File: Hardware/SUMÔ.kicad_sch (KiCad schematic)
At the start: 17 parts, among them M1 Motor_DC, M2 Motor_DC, SW1 SW_DPST_x2

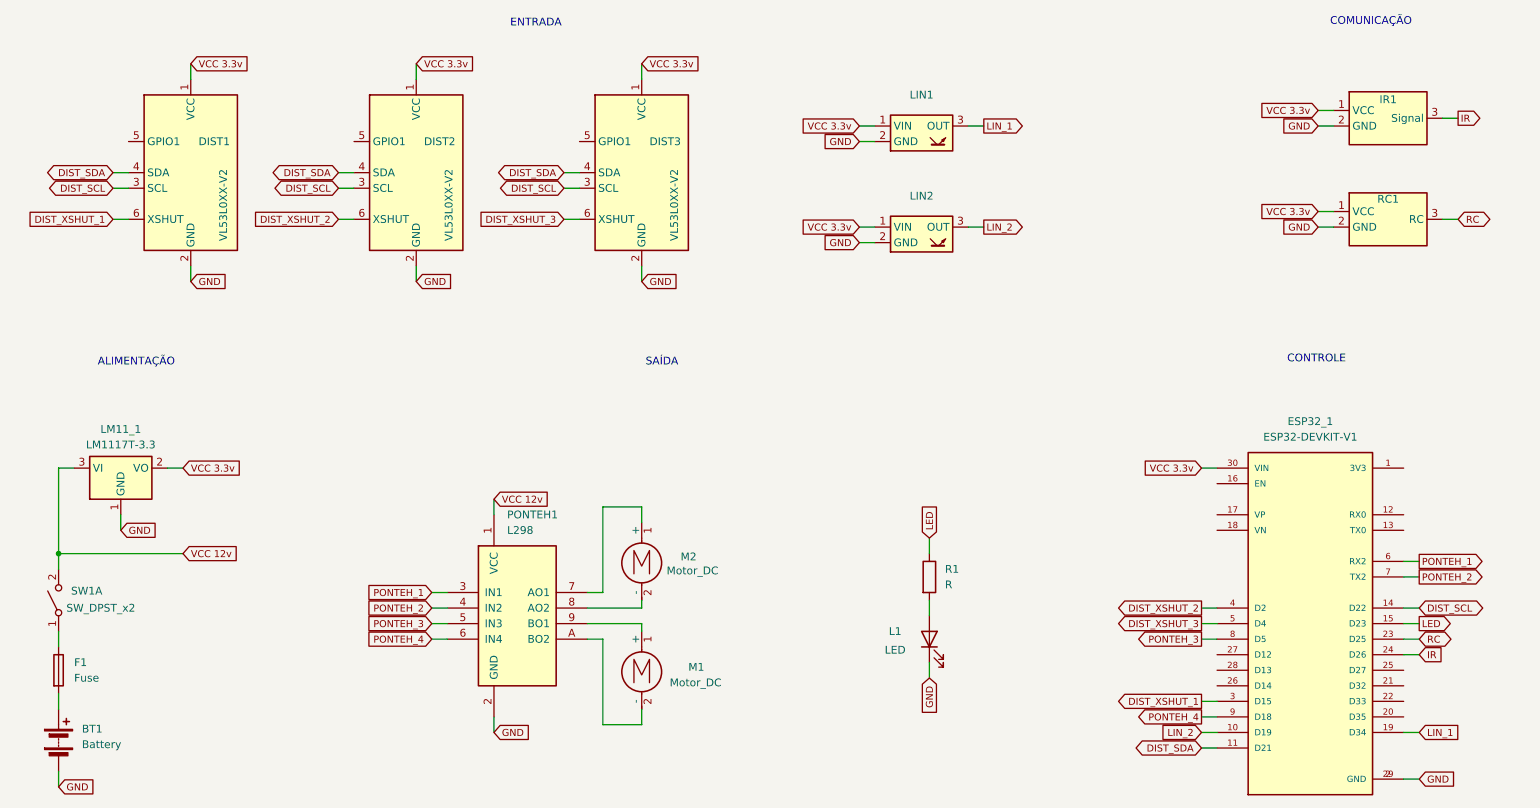
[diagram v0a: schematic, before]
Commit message: V3: (circuito) update Hardware
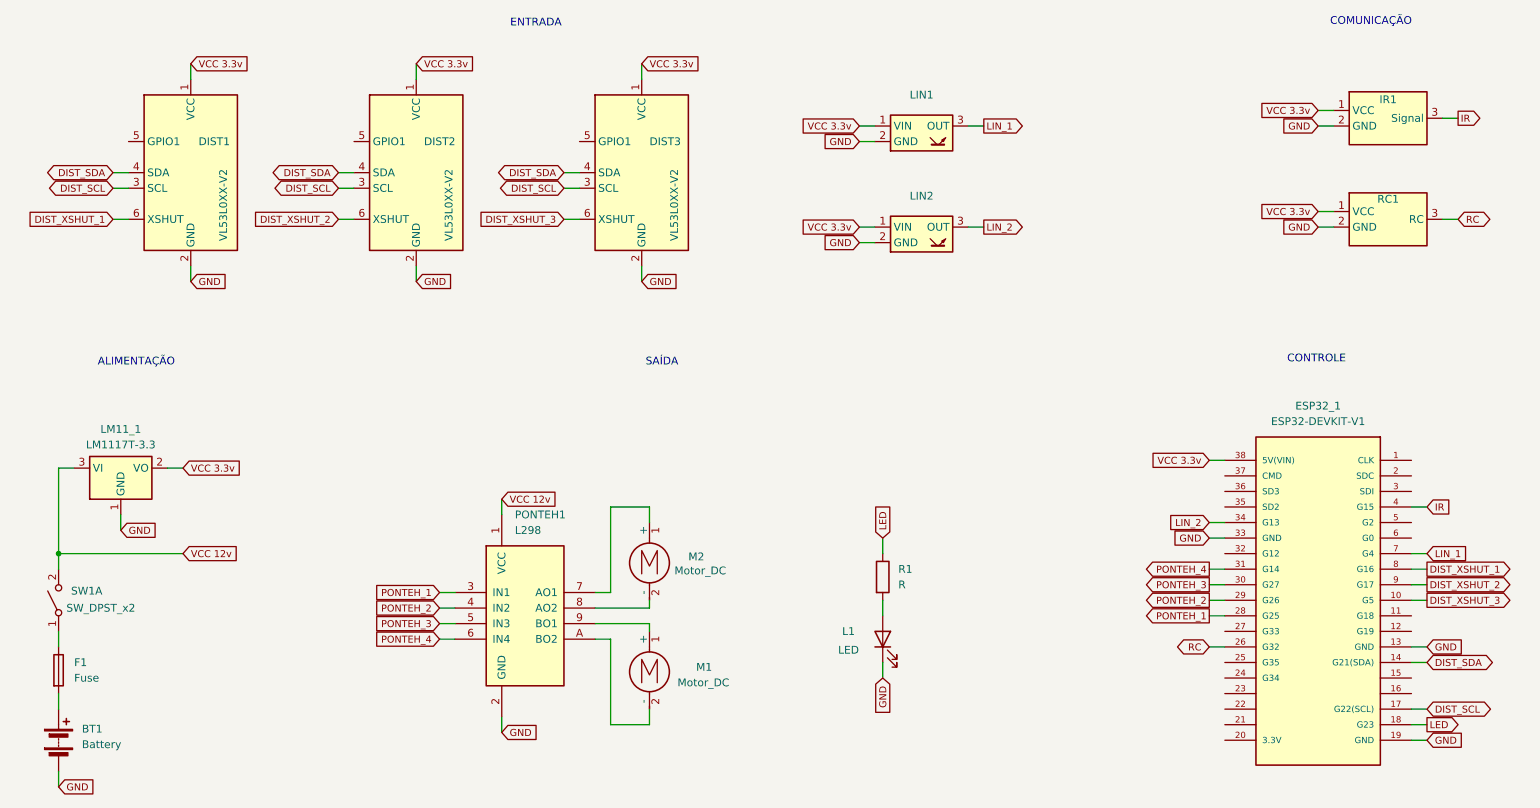
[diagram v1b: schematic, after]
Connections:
- net DIST_SCL: now also ESP32_1.17 (G22(SCL)); no longer ESP32_1.14 (D22)
- net DIST_SDA: now also ESP32_1.14 (G21(SDA)); no longer ESP32_1.11 (D21)
- net DIST_XSHUT_1: now also ESP32_1.8 (G16); no longer ESP32_1.3 (D15)
- net DIST_XSHUT_2: now also ESP32_1.9 (G17); no longer ESP32_1.4 (D2)
- net DIST_XSHUT_3: now also ESP32_1.10 (G5); no longer ESP32_1.5 (D4)
- net GND: now also ESP32_1.13 (GND), ESP32_1.19 (GND), ESP32_1.33 (GND); no longer ESP32_1.2 (GND), ESP32_1.29 (GND)
- net IR: now also ESP32_1.4 (G15); no longer ESP32_1.24 (D26)
- net LED: now also ESP32_1.18 (G23); no longer ESP32_1.15 (D23)
- net LIN_1: now also ESP32_1.7 (G4); no longer ESP32_1.19 (D34)
- net LIN_2: now also ESP32_1.34 (G13); no longer ESP32_1.10 (D19)
- net PONTEH_1: now also ESP32_1.28 (G25); no longer ESP32_1.6 (RX2)
- net PONTEH_2: now also ESP32_1.29 (G26); no longer ESP32_1.7 (TX2)
- net PONTEH_3: now also ESP32_1.30 (G27); no longer ESP32_1.8 (D5)
- net PONTEH_4: now also ESP32_1.31 (G14); no longer ESP32_1.9 (D18)
- net RC: now also ESP32_1.26 (G32); no longer ESP32_1.23 (D25)
- net VCC 3.3v: now also ESP32_1.38 (5V(VIN)); no longer ESP32_1.30 (VIN)
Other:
- moved on the sheet: L1, M1, M2, PONTEH1, R1
